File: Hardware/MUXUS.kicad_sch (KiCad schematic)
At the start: 124 parts, among them J1 USB_C_Receptacle_USB2.0, J10 USB_A, J2 USB_B, J3 USB_A, J4 USB_B, J5 USB_A, J6 STDC14, J7 SWD, J8 VCP, J9 USB_B, SW1 USER, SW2 RESET, U1 USBLC6-4SC6, U10 AP2151W, U11 AOZ1212AI, U12 USBLC6-2SC6, U13 USBLC6-2SC6, U14 AP2151W, U2 USB2504A-JT, U3 USBLC6-2SC6, U4 USBLC6-2SC6, U5 AP2151W, U6 TS3USBCA420RSVR, U7 STM32G441KBU6, U8 USBLC6-2SC6, U9 USBLC6-2SC6, Y1 ATS240C

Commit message: AMOGUS
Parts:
- SYM1: footprint AMOGUS:SUS -> leptunKicadLib:AMOGUS
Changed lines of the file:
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@@
     )
     (property "Value" "AMOGUS" (id 1) (at 64.643 263.398 0))
-    (property "Footprint" "AMOGUS:SUS" (id 2) (at 64.643 262.128 0)
+    (property "Footprint" "leptunKicadLib:AMOGUS" (id 2) (at 64.643 262.128 0)
       (effects (font (size 1.27 1.27)) hide)
     )
@@
     )
     (path "/00000000-0000-0000-0000-0000615445ff"
-      (reference "SYM1") (unit 1) (value "AMOGUS") (footprint "AMOGUS:SUS")
+      (reference "SYM1") (unit 1) (value "AMOGUS") (footprint "leptunKicadLib:AMOGUS")
     )
     (path "/00000000-0000-0000-0000-000061a4e349"

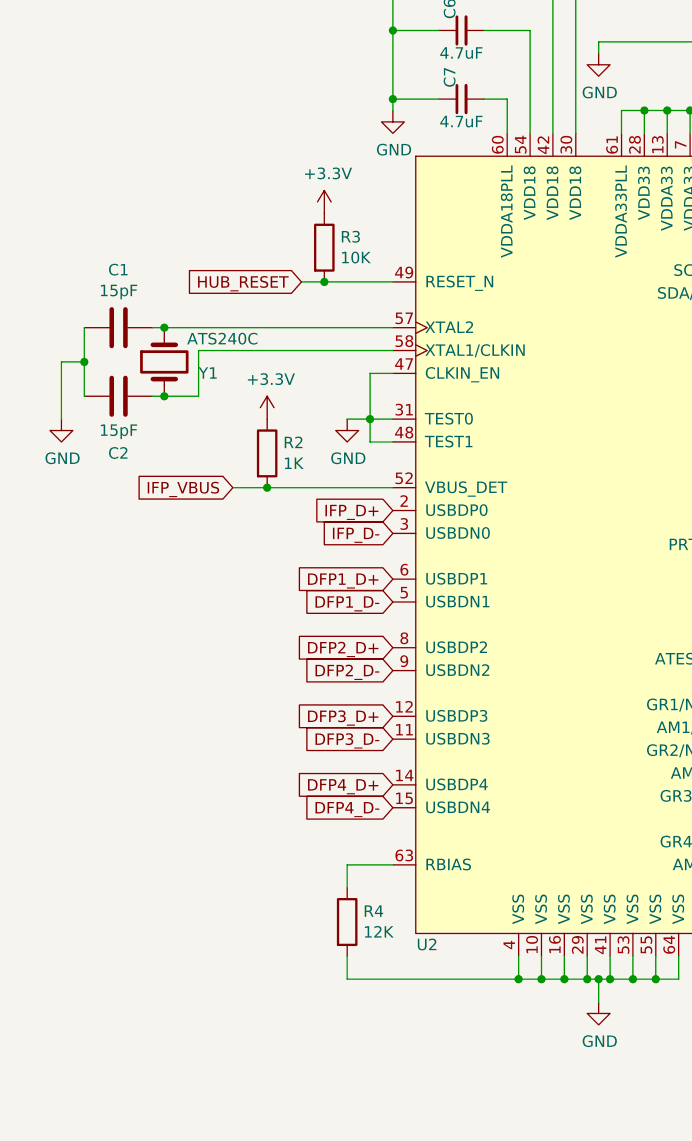
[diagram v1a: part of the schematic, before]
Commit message: USB2504A-JT
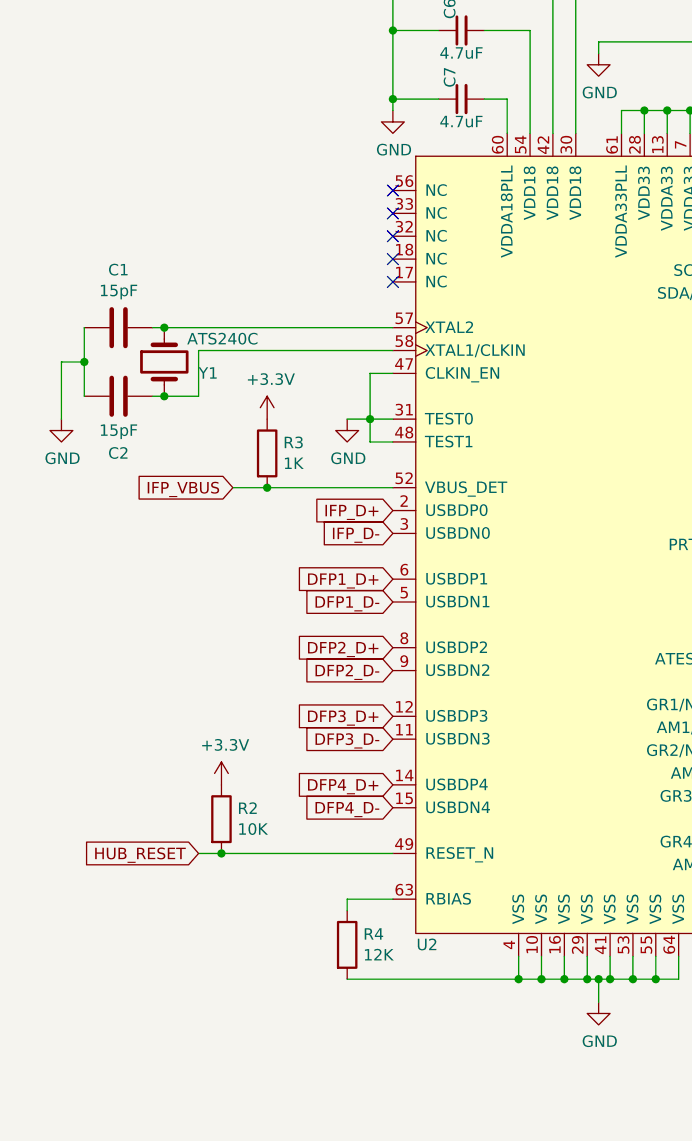
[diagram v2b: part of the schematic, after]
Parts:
- U2: symbol USB2504A-JT:USB2504A-JT -> leptunKicadLib:USB2504A-JT
- renumbered R3 to R2, R2 to R3
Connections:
- no-connect marks 9 -> 14
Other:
- moved on the sheet: R2, R4
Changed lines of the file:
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@@
   (junction (at 35.56 158.75) (diameter 0) (color 0 0 0 0))
   (junction (at 35.56 166.37) (diameter 0) (color 0 0 0 0))
+  (junction (at 41.91 217.17) (diameter 0) (color 0 0 0 0))
   (junction (at 46.99 176.53) (diameter 0) (color 0 0 0 0))
   (junction (at 52.07 41.91) (diameter 0) (color 0 0 0 0))
   (junction (at 52.07 46.99) (diameter 0) (color 0 0 0 0))
-  (junction (at 53.34 153.67) (diameter 0) (color 0 0 0 0))
   (junction (at 54.61 41.91) (diameter 0) (color 0 0 0 0))
   (junction (at 57.15 33.02) (diameter 0) (color 0 0 0 0))
@@
   (no_connect (at 50.8 55.88))
   (no_connect (at 50.8 58.42))
+  (no_connect (at 60.96 143.51))
+  (no_connect (at 60.96 146.05))
+  (no_connect (at 60.96 148.59))
+  (no_connect (at 60.96 151.13))
+  (no_connect (at 60.96 153.67))
   (no_connect (at 106.68 160.02))
   (no_connect (at 106.68 162.56))
@@
     (stroke (width 0) (type default) (color 0 0 0 0))
   )
+  (wire (pts (xy 41.91 217.17) (xy 39.37 217.17))
+    (stroke (width 0) (type default) (color 0 0 0 0))
+  )
+  (wire (pts (xy 41.91 217.17) (xy 60.96 217.17))
+    (stroke (width 0) (type default) (color 0 0 0 0))
+  )
   (wire (pts (xy 43.18 176.53) (xy 46.99 176.53))
     (stroke (width 0) (type default) (color 0 0 0 0))
@@
     (stroke (width 0) (type default) (color 0 0 0 0))
   )
-  (wire (pts (xy 53.34 153.67) (xy 50.8 153.67))
-    (stroke (width 0) (type default) (color 0 0 0 0))
-  )
-  (wire (pts (xy 53.34 153.67) (xy 60.96 153.67))
-    (stroke (width 0) (type default) (color 0 0 0 0))
-  )
   (wire (pts (xy 54.61 41.91) (xy 82.55 41.91))
     (stroke (width 0) (type default) (color 0 0 0 0))
@@
     (stroke (width 0) (type default) (color 0 0 0 0))
   )
-  (wire (pts (xy 55.88 218.44) (xy 60.96 218.44))
-    (stroke (width 0) (type default) (color 0 0 0 0))
-  )
-  (wire (pts (xy 55.88 220.98) (xy 55.88 218.44))
-    (stroke (width 0) (type default) (color 0 0 0 0))
-  )
-  (wire (pts (xy 55.88 228.6) (xy 55.88 231.14))
+  (wire (pts (xy 55.88 222.25) (xy 55.88 223.52))
     (stroke (width 0) (type default) (color 0 0 0 0))
   )
@@
     (stroke (width 0) (type default) (color 0 0 0 0))
   )
+  (wire (pts (xy 60.96 222.25) (xy 55.88 222.25))
+    (stroke (width 0) (type default) (color 0 0 0 0))
+  )
   (wire (pts (xy 67.31 27.94) (xy 50.8 27.94))
     (stroke (width 0) (type default) (color 0 0 0 0))
@@
     (stroke (width 0) (type default) (color 0 0 0 0))
   )
-  (global_label "IFP_VBUS" (shape input) (at 43.18 176.53 180) (fields_autoplaced)
+  (global_label "HUB_RESET" (shape input) (at 39.37 217.17 180) (fields_autoplaced)
     (effects (font (size 1.27 1.27)) (justify right))
-    (property "Intersheet References" "${INTERSHEET_REFS}" (id 0) (at 0 0 0)
+    (property "Intersheet References" "${INTERSHEET_REFS}" (id 0) (at -11.43 63.5 0)
       (effects (font (size 1.27 1.27)) hide)
     )
   )
-  (global_label "HUB_RESET" (shape input) (at 50.8 153.67 180) (fields_autoplaced)
+  (global_label "IFP_VBUS" (shape input) (at 43.18 176.53 180) (fields_autoplaced)
     (effects (font (size 1.27 1.27)) (justify right))
     (property "Intersheet References" "${INTERSHEET_REFS}" (id 0) (at 0 0 0)
@@
     )
   )
-  (symbol (lib_id "power:+3.3V") (at 46.99 168.91 0) (unit 1)
+  (symbol (lib_id "power:+3.3V") (at 41.91 209.55 0) (unit 1)
     (in_bom yes) (on_board yes)
-    (property "Reference" "#PWR04" (id 0) (at 46.99 172.72 0)
+    (property "Reference" "#PWR04" (id 0) (at 41.91 213.36 0)
       (effects (font (size 1.27 1.27)) hide)
     )
-    (property "Value" "+3.3V" (id 1) (at 47.371 164.5158 0))
-    (property "Footprint" "" (id 2) (at 46.99 168.91 0)
+    (property "Value" "+3.3V" (id 1) (at 42.291 205.1558 0))
+    (property "Footprint" "" (id 2) (at 41.91 209.55 0)
       (effects (font (size 1.27 1.27)) hide)
     )
-    (property "Datasheet" "" (id 3) (at 46.99 168.91 0)
+    (property "Datasheet" "" (id 3) (at 41.91 209.55 0)
       (effects (font (size 1.27 1.27)) hide)
     )
     (pin "1")
   )
-  (symbol (lib_id "power:+3.3V") (at 53.34 146.05 0) (unit 1)
+  (symbol (lib_id "power:+3.3V") (at 46.99 168.91 0) (unit 1)
     (in_bom yes) (on_board yes)
-    (property "Reference" "#PWR05" (id 0) (at 53.34 149.86 0)
+    (property "Reference" "#PWR05" (id 0) (at 46.99 172.72 0)
       (effects (font (size 1.27 1.27)) hide)
     )
-    (property "Value" "+3.3V" (id 1) (at 53.721 141.6558 0))
-    (property "Footprint" "" (id 2) (at 53.34 146.05 0)
+    (property "Value" "+3.3V" (id 1) (at 47.371 164.5158 0))
+    (property "Footprint" "" (id 2) (at 46.99 168.91 0)
       (effects (font (size 1.27 1.27)) hide)
     )
-    (property "Datasheet" "" (id 3) (at 53.34 146.05 0)
+    (property "Datasheet" "" (id 3) (at 46.99 168.91 0)
       (effects (font (size 1.27 1.27)) hide)
     )
@@
     (pin "2")
   )
-  (symbol (lib_id "Device:R") (at 46.99 172.72 0) (unit 1)
+  (symbol (lib_id "Device:R") (at 41.91 213.36 0) (unit 1)
     (in_bom yes) (on_board yes)
-    (property "Reference" "R2" (id 0) (at 48.768 171.5516 0)
+    (property "Reference" "R2" (id 0) (at 43.688 212.1916 0)
       (effects (font (size 1.27 1.27)) (justify left))
     )
-    (property "Value" "1K" (id 1) (at 48.768 173.863 0)
+    (property "Value" "10K" (id 1) (at 43.688 214.503 0)
       (effects (font (size 1.27 1.27)) (justify left))
     )
-    (property "Footprint" "Resistor_SMD:R_1206_3216Metric" (id 2) (at 45.212 172.72 90)
+    (property "Footprint" "Resistor_SMD:R_1206_3216Metric" (id 2) (at 40.132 213.36 90)
       (effects (font (size 1.27 1.27)) hide)
     )
-    (property "Datasheet" "~" (id 3) (at 46.99 172.72 0)
+    (property "Datasheet" "~" (id 3) (at 41.91 213.36 0)
       (effects (font (size 1.27 1.27)) hide)
     )
@@
     (pin "2")
   )
-  (symbol (lib_id "Device:R") (at 53.34 149.86 0) (unit 1)
+  (symbol (lib_id "Device:R") (at 46.99 172.72 0) (unit 1)
     (in_bom yes) (on_board yes)
-    (property "Reference" "R3" (id 0) (at 55.118 148.6916 0)
+    (property "Reference" "R3" (id 0) (at 48.768 171.5516 0)
       (effects (font (size 1.27 1.27)) (justify left))
     )
-    (property "Value" "10K" (id 1) (at 55.118 151.003 0)
+    (property "Value" "1K" (id 1) (at 48.768 173.863 0)
       (effects (font (size 1.27 1.27)) (justify left))
     )
-    (property "Footprint" "Resistor_SMD:R_1206_3216Metric" (id 2) (at 51.562 149.86 90)
+    (property "Footprint" "Resistor_SMD:R_1206_3216Metric" (id 2) (at 45.212 172.72 90)
       (effects (font (size 1.27 1.27)) hide)
     )
-    (property "Datasheet" "~" (id 3) (at 53.34 149.86 0)
+    (property "Datasheet" "~" (id 3) (at 46.99 172.72 0)
       (effects (font (size 1.27 1.27)) hide)
     )
@@
     (pin "2")
   )
-  (symbol (lib_id "Device:R") (at 55.88 224.79 0) (unit 1)
+  (symbol (lib_id "Device:R") (at 55.88 227.33 0) (unit 1)
     (in_bom yes) (on_board yes)
-    (property "Reference" "R4" (id 0) (at 57.658 223.6216 0)
+    (property "Reference" "R4" (id 0) (at 57.658 226.1616 0)
       (effects (font (size 1.27 1.27)) (justify left))
     )
-    (property "Value" "12K" (id 1) (at 57.658 225.933 0)
+    (property "Value" "12K" (id 1) (at 57.658 228.473 0)
       (effects (font (size 1.27 1.27)) (justify left))
     )
-    (property "Footprint" "Resistor_SMD:R_1206_3216Metric" (id 2) (at 54.102 224.79 90)
+    (property "Footprint" "Resistor_SMD:R_1206_3216Metric" (id 2) (at 54.102 227.33 90)
       (effects (font (size 1.27 1.27)) hide)
     )
-    (property "Datasheet" "~" (id 3) (at 55.88 224.79 0)
+    (property "Datasheet" "~" (id 3) (at 55.88 227.33 0)
       (effects (font (size 1.27 1.27)) hide)
     )
@@
     (pin "S1")
   )
-  (symbol (lib_id "USB2504A-JT:USB2504A-JT") (at 83.82 182.88 0) (unit 1)
+  (symbol (lib_id "leptunKicadLib:USB2504A-JT") (at 83.82 182.88 0) (unit 1)
     (in_bom yes) (on_board yes)
     (property "Reference" "U2" (id 0) (at 64.77 227.33 0))
@@
     (pin "15")
     (pin "16")
+    (pin "17")
+    (pin "18")
     (pin "19")
     (pin "2")
@@
     (pin "30")
     (pin "31")
+    (pin "32")
+    (pin "33")
     (pin "34")
     (pin "35")
@@
     (pin "54")
     (pin "55")
+    (pin "56")
     (pin "57")
     (pin "58")
@@
       (reference "#PWR03") (unit 1) (value "GND") (footprint "")
     )
-    (path "/00000000-0000-0000-0000-000061909e24"
+    (path "/00000000-0000-0000-0000-000061d2f1f1"
       (reference "#PWR04") (unit 1) (value "+3.3V") (footprint "")
     )
-    (path "/00000000-0000-0000-0000-000061d2f1f1"
+    (path "/00000000-0000-0000-0000-000061909e24"
       (reference "#PWR05") (unit 1) (value "+3.3V") (footprint "")
     )
@@
       (reference "R1") (unit 1) (value "330R") (footprint "Resistor_SMD:R_0805_2012Metric")
     )
-    (path "/00000000-0000-0000-0000-0000619095ed"
-      (reference "R2") (unit 1) (value "1K") (footprint "Resistor_SMD:R_1206_3216Metric")
-    )
     (path "/00000000-0000-0000-0000-000061d0b1ed"
-      (reference "R3") (unit 1) (value "10K") (footprint "Resistor_SMD:R_1206_3216Metric")
+      (reference "R2") (unit 1) (value "10K") (footprint "Resistor_SMD:R_1206_3216Metric")
+    )
+    (path "/00000000-0000-0000-0000-0000619095ed"
+      (reference "R3") (unit 1) (value "1K") (footprint "Resistor_SMD:R_1206_3216Metric")
     )
     (path "/00000000-0000-0000-0000-000061ac4413"

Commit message: TS3USBCA420RSVR
.
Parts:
- U6: footprint TS3USBCA420RSVR:TS3USBCA420RSVR -> leptunKicadLib:TS3USBCA420RSVR; symbol TS3USBCA420RSVR:TS3USBCA420RSVR -> leptunKicadLib:TS3USBCA420RSVR
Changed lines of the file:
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@@
     (pin "8")
   )
-  (symbol (lib_id "TS3USBCA420RSVR:TS3USBCA420RSVR") (at 201.93 243.84 0) (unit 1)
+  (symbol (lib_id "leptunKicadLib:TS3USBCA420RSVR") (at 201.93 243.84 0) (unit 1)
     (in_bom yes) (on_board yes)
     (property "Reference" "U6" (id 0) (at 201.93 224.409 0))
     (property "Value" "TS3USBCA420RSVR" (id 1) (at 201.93 226.7204 0))
-    (property "Footprint" "TS3USBCA420RSVR:TS3USBCA420RSVR" (id 2) (at 219.71 278.13 0)
+    (property "Footprint" "leptunKicadLib:TS3USBCA420RSVR" (id 2) (at 219.71 278.13 0)
       (effects (font (size 1.27 1.27)) hide)
     )
@@
     )
     (path "/00000000-0000-0000-0000-0000614c3d23"
-      (reference "U6") (unit 1) (value "TS3USBCA420RSVR") (footprint "TS3USBCA420RSVR:TS3USBCA420RSVR")
+      (reference "U6") (unit 1) (value "TS3USBCA420RSVR") (footprint "leptunKicadLib:TS3USBCA420RSVR")
     )
     (path "/00000000-0000-0000-0000-00006191bd86"

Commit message: FTSH-107-01-L-DV-K-A
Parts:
- J6: footprint FTSH-107-01-L-DV-K-A:FTSH-107-01-L-DV-K-A -> leptunKicadLib:FTSH-107-01-L-DV-K-A
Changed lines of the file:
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@@
     (property "Reference" "J6" (id 0) (at 267.97 204.0382 0))
     (property "Value" "STDC14" (id 1) (at 267.97 206.3496 0))
-    (property "Footprint" "FTSH-107-01-L-DV-K-A:FTSH-107-01-L-DV-K-A" (id 2) (at 266.7 217.17 0)
+    (property "Footprint" "leptunKicadLib:FTSH-107-01-L-DV-K-A" (id 2) (at 266.7 217.17 0)
       (effects (font (size 1.27 1.27)) hide)
     )
@@
     )
     (path "/00000000-0000-0000-0000-000061f739e3"
-      (reference "J6") (unit 1) (value "STDC14") (footprint "FTSH-107-01-L-DV-K-A:FTSH-107-01-L-DV-K-A")
+      (reference "J6") (unit 1) (value "STDC14") (footprint "leptunKicadLib:FTSH-107-01-L-DV-K-A")
     )
     (path "/00000000-0000-0000-0000-0000615b40a3"
